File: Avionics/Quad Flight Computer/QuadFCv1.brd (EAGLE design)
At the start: 49.5 x 49.5 mm, 122 parts, among them J2 1050270001, Q1 DMP2035U, Q2 DMP2035U, Q3 DMP2035U, SW1 PTS635VL31-VERT, U1 TM4C123GH6PZ, U10 LTC4412, U11 AP7215-33YG-13, U2 74LVC4245APW, U3 ATMEGA32U2-MU, U5 INVESENSE_MPU-6000, U6 HMC5883LSMD, U7 MS5611-01BA, U8 74AUP1G19GW, U9 S25FL127S, X1 HWB, Y1 32.768KHZ, Y2 AWSCR-20.00CW-T, Y3 PRQC16.00SR5010X000

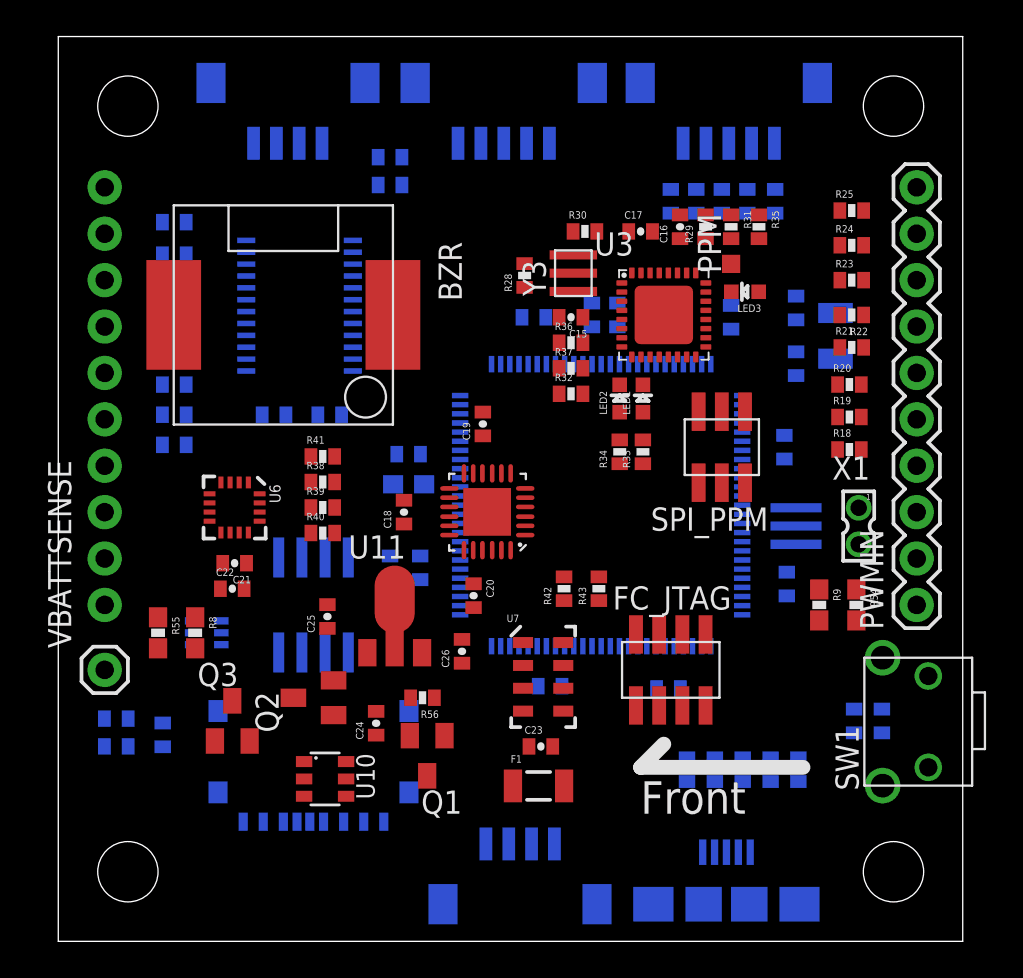
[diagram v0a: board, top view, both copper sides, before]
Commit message: Minor updates.
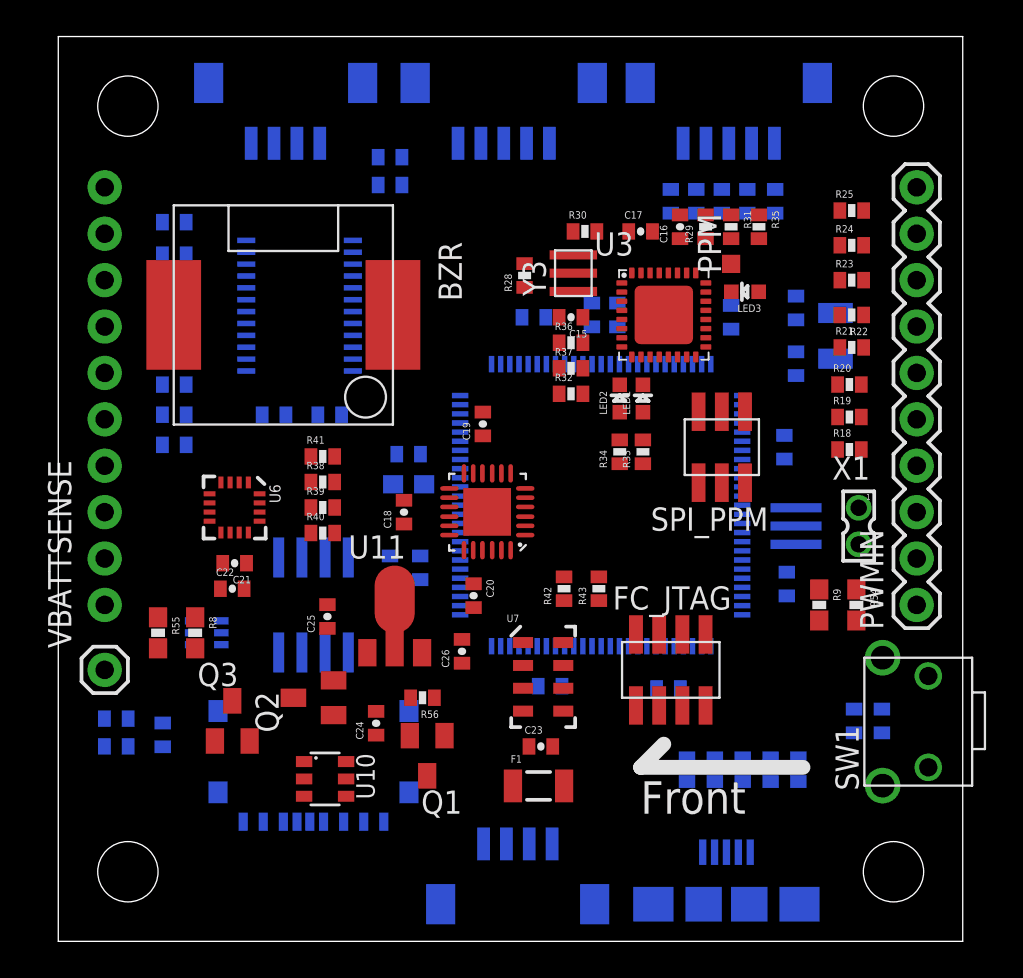
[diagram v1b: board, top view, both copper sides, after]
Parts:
- moved GPS 2.65 mm to (12.4, 43.7)
- moved I2C 2.59 mm to (25.1, 5.33)
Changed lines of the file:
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@@
 <layer number="220" name="220bmp" color="21" fill="1" visible="no" active="no"/>
 <layer number="221" name="221bmp" color="22" fill="1" visible="no" active="no"/>
+<layer number="222" name="222bmp" color="7" fill="1" visible="yes" active="yes"/>
 <layer number="223" name="223bmp" color="24" fill="1" visible="no" active="no"/>
 <layer number="224" name="224bmp" color="25" fill="1" visible="no" active="no"/>
@@
 <element name="R50" library="QuadFCv1" package="0402-RES" value="10k" x="37.719" y="40.513" rot="MR270"/>
 <element name="R51" library="QuadFCv1" package="0402-RES" value="10k" x="39.243" y="40.513" rot="MR270"/>
-<element name="I2C" library="QuadFCv1" package="DF13_4POS" value="" x="24.638" y="2.794" rot="MR180"/>
-<element name="GPS" library="QuadFCv1" package="DF13_4POS" value="" x="13.208" y="46.228" rot="MR0"/>
+<element name="I2C" library="QuadFCv1" package="DF13_4POS" value="" x="25.146" y="5.334" rot="MR180"/>
+<element name="GPS" library="QuadFCv1" package="DF13_4POS" value="" x="12.446" y="43.688" rot="MR0"/>
 <element name="R52" library="QuadFCv1" package="0402-RES" value="0" x="18.161" y="41.402" rot="MR180"/>
 <element name="R53" library="QuadFCv1" package="0402-RES" value="DNP" x="18.161" y="42.926" rot="MR180"/>
@@
 <wire x1="8.902" y1="25.119" x2="9.902" y2="25.119" width="0" layer="19" extent="1-1"/>
 <wire x1="11.022" y1="22.999" x2="9.902" y2="25.119" width="0" layer="19" extent="1-1"/>
-<wire x1="23.408" y1="5.334" x2="25.766" y2="10.668" width="0" layer="19" extent="1-16"/>
+<wire x1="23.281" y1="5.334" x2="25.766" y2="10.668" width="0" layer="19" extent="1-16"/>
 <wire x1="7.328" y1="16.891" x2="11.022" y2="22.999" width="0" layer="19" extent="1-16"/>
 <wire x1="12.065" y1="15.815" x2="7.328" y2="16.891" width="0" layer="19" extent="16-16"/>
@@
 <wire x1="35.433" y1="12.9159" x2="34.163" y2="12.9159" width="0" layer="19" extent="1-1"/>
 <wire x1="33.218" y1="16.156" x2="32.751" y2="13.843" width="0" layer="19" extent="16-16"/>
-<wire x1="27.158" y1="5.334" x2="27.066" y2="10.668" width="0" layer="19" extent="1-16"/>
+<wire x1="27.031" y1="5.334" x2="27.066" y2="10.668" width="0" layer="19" extent="1-16"/>
 <wire x1="8.928" y1="16.891" x2="14.732" y2="18.43" width="0" layer="19" extent="1-16"/>
 <wire x1="9.002" y1="20.701" x2="8.928" y2="16.891" width="0" layer="19" extent="1-16"/>
@@
 <wire x1="10.2902" y1="37.723" x2="12.461" y2="28.829" width="0" layer="19" extent="16-16"/>
 <wire x1="10.2902" y1="38.373" x2="10.2902" y2="37.723" width="0" layer="19" extent="16-16"/>
-<wire x1="10.688" y1="43.688" x2="10.2902" y2="38.373" width="0" layer="19" extent="16-16"/>
+<wire x1="10.561" y1="43.688" x2="10.2902" y2="38.373" width="0" layer="19" extent="16-16"/>
 <wire x1="16.1258" y1="38.373" x2="10.2902" y2="38.373" width="0" layer="19" extent="16-16"/>
 <wire x1="21.884" y1="43.688" x2="16.1258" y2="38.373" width="0" layer="19" extent="16-16"/>
@@
 <contactref element="R53" pad="1"/>
 <wire x1="17.511" y1="42.926" x2="17.511" y2="41.402" width="0" layer="19" extent="16-16"/>
-<wire x1="14.438" y1="43.688" x2="17.511" y2="42.926" width="0" layer="19" extent="16-16"/>
+<wire x1="14.311" y1="43.688" x2="17.511" y2="42.926" width="0" layer="19" extent="16-16"/>
 </signal>
 <signal name="GPS_TX">

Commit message: Updated part references
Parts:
- GPS, I2C: device QuadFCv1:DF13_4POS -> QuadFCv1:DF13A-4P-1.25H
- ISENSE, RADIO1: device QuadFCv1:DF13_5POS -> QuadFCv1:DF13A-5P-1.25H
- LED1, LED2, LED3: device QuadFCv1:SPARKFUN_LED-0603 -> QuadFCv1:LED-0603
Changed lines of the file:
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@@
 <layer number="23" name="tOrigins" color="15" fill="1" visible="yes" active="yes"/>
 <layer number="24" name="bOrigins" color="15" fill="1" visible="yes" active="yes"/>
-<layer number="25" name="tNames" color="7" fill="1" visible="no" active="yes"/>
-<layer number="26" name="bNames" color="7" fill="1" visible="no" active="yes"/>
+<layer number="25" name="tNames" color="7" fill="1" visible="yes" active="yes"/>
+<layer number="26" name="bNames" color="7" fill="1" visible="yes" active="yes"/>
 <layer number="27" name="tValues" color="7" fill="1" visible="no" active="yes"/>
 <layer number="28" name="bValues" color="7" fill="1" visible="no" active="yes"/>
@@
 <layer number="37" name="tTest" color="7" fill="1" visible="no" active="yes"/>
 <layer number="38" name="bTest" color="7" fill="1" visible="no" active="yes"/>
-<layer number="39" name="tKeepout" color="4" fill="11" visible="yes" active="yes"/>
-<layer number="40" name="bKeepout" color="1" fill="11" visible="yes" active="yes"/>
-<layer number="41" name="tRestrict" color="4" fill="10" visible="yes" active="yes"/>
-<layer number="42" name="bRestrict" color="1" fill="10" visible="yes" active="yes"/>
-<layer number="43" name="vRestrict" color="2" fill="10" visible="yes" active="yes"/>
+<layer number="39" name="tKeepout" color="4" fill="11" visible="no" active="yes"/>
+<layer number="40" name="bKeepout" color="1" fill="11" visible="no" active="yes"/>
+<layer number="41" name="tRestrict" color="4" fill="10" visible="no" active="yes"/>
+<layer number="42" name="bRestrict" color="1" fill="10" visible="no" active="yes"/>
+<layer number="43" name="vRestrict" color="2" fill="10" visible="no" active="yes"/>
 <layer number="44" name="Drills" color="7" fill="1" visible="no" active="yes"/>
-<layer number="45" name="Holes" color="7" fill="1" visible="yes" active="yes"/>
+<layer number="45" name="Holes" color="7" fill="1" visible="no" active="yes"/>
 <layer number="46" name="Milling" color="3" fill="1" visible="no" active="yes"/>
 <layer number="47" name="Measures" color="7" fill="1" visible="no" active="yes"/>
-<layer number="48" name="Document" color="7" fill="1" visible="yes" active="yes"/>
-<layer number="49" name="Reference" color="7" fill="1" visible="yes" active="yes"/>
+<layer number="48" name="Document" color="7" fill="1" visible="no" active="yes"/>
+<layer number="49" name="Reference" color="7" fill="1" visible="no" active="yes"/>
 <layer number="50" name="dxf" color="7" fill="1" visible="no" active="no"/>
 <layer number="51" name="tDocu" color="7" fill="1" visible="yes" active="yes"/>
@@
 <layer number="144" name="Drill_legend" color="7" fill="1" visible="no" active="yes"/>
 <layer number="151" name="HeatSink" color="7" fill="1" visible="no" active="yes"/>
-<layer number="199" name="Contour" color="7" fill="1" visible="yes" active="yes"/>
+<layer number="199" name="Contour" color="7" fill="1" visible="no" active="yes"/>
 <layer number="200" name="200bmp" color="1" fill="10" visible="no" active="yes"/>
 <layer number="201" name="201bmp" color="2" fill="10" visible="no" active="yes"/>
@@
 <element name="C15" library="QuadFCv1" package="0402-CAP" value=".1uF" x="28.067" y="34.163" rot="R180"/>
 <element name="C16" library="QuadFCv1" package="0402-CAP" value="1uF" x="34.036" y="39.116" rot="R90"/>
-<element name="LED1" library="QuadFCv1" package="SPARKFUN_LED-0603" value="RED" x="32.004" y="29.718"/>
-<element name="LED2" library="QuadFCv1" package="SPARKFUN_LED-0603" value="ORANGE" x="30.734" y="29.718"/>
+<element name="LED1" library="QuadFCv1" package="LED-0603" value="RED" x="32.004" y="29.718"/>
+<element name="LED2" library="QuadFCv1" package="LED-0603" value="ORANGE" x="30.734" y="29.718"/>
 <element name="R33" library="QuadFCv1" package="0402-RES" value="1k" x="32.004" y="26.797" rot="R90"/>
 <element name="R34" library="QuadFCv1" package="0402-RES" value="1k" x="30.734" y="26.797" rot="R90"/>
@@
 <element name="R37" library="QuadFCv1" package="0402-RES" value="1k" x="28.067" y="31.369"/>
 <element name="R35" library="QuadFCv1" package="0402-RES" value="1k" x="38.354" y="39.116" rot="R270"/>
-<element name="LED3" library="QuadFCv1" package="SPARKFUN_LED-0603" value="GREEN" x="37.592" y="35.56" rot="R90"/>
+<element name="LED3" library="QuadFCv1" package="LED-0603" value="GREEN" x="37.592" y="35.56" rot="R90"/>
 <element name="F1" library="QuadFCv1" package="PTC-1206" value="500mA" x="26.289" y="8.509"/>
 <element name="Y3" library="QuadFCv1" package="PRQC16.00SR5010X000" value="PRQC16.00SR5010X000" x="28.194" y="36.576" rot="R90"/>
@@
 <element name="J2" library="QuadFCv1" package="1050270001" value="1050270001" x="13.97" y="13.208" rot="MR0"/>
 <element name="FC_JTAG" library="QuadFCv1" package="2X4_SMT-0.05" value="M04X2SMT-0.05" x="32.893" y="14.859"/>
-<element name="ISENSE" library="QuadFCv1" package="DF13_5POS" value="" x="36.703" y="43.688" rot="MR0"/>
+<element name="ISENSE" library="QuadFCv1" package="DF13A-5P-1.25H" value="" x="36.703" y="43.688" rot="MR0"/>
 <element name="VBATTSENSE" library="QuadFCv1" package="1X01" value="M01PTH" x="2.54" y="14.859" rot="R90"/>
 <element name="R44" library="QuadFCv1" package="0402-RES" value="120K" x="3.175" y="12.192" rot="MR0"/>
@@
 <element name="R50" library="QuadFCv1" package="0402-RES" value="10k" x="37.719" y="40.513" rot="MR270"/>
 <element name="R51" library="QuadFCv1" package="0402-RES" value="10k" x="39.243" y="40.513" rot="MR270"/>
-<element name="I2C" library="QuadFCv1" package="DF13_4POS" value="" x="25.146" y="5.334" rot="MR180"/>
-<element name="GPS" library="QuadFCv1" package="DF13_4POS" value="" x="12.446" y="43.688" rot="MR0"/>
+<element name="I2C" library="QuadFCv1" package="DF13A-4P-1.25H" value="" x="25.146" y="5.334" rot="MR180"/>
+<element name="GPS" library="QuadFCv1" package="DF13A-4P-1.25H" value="" x="12.446" y="43.688" rot="MR0"/>
 <element name="R52" library="QuadFCv1" package="0402-RES" value="0" x="18.161" y="41.402" rot="MR180"/>
 <element name="R53" library="QuadFCv1" package="0402-RES" value="DNP" x="18.161" y="42.926" rot="MR180"/>
@@
 <element name="C25" library="QuadFCv1" package="0402-CAP" value="1u" x="14.732" y="17.78" rot="R90"/>
 <element name="C26" library="QuadFCv1" package="0402-CAP" value="1u" x="22.098" y="15.875" rot="R90"/>
-<element name="RADIO1" library="QuadFCv1" package="DF13_5POS" value="" x="24.384" y="43.688" rot="MR0"/>
+<element name="RADIO1" library="QuadFCv1" package="DF13A-5P-1.25H" value="" x="24.384" y="43.688" rot="MR0"/>
 <element name="U12" library="QuadFCv1" package="USB-AB-MICRO-SMD" value="" x="36.576" y="2.032" rot="MR90"/>
 <element name="SW1" library="QuadFCv1" package="PTS635VL31" value="PTS635VL31-VERT" x="47.625" y="9.525" rot="R90"/>
